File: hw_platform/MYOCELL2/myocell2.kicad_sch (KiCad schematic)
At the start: 22 parts, among them J1 Conn_01x16, J2 Conn_01x16, U1 ESP32-WROOM-32, U2 OPA340NA, U3 ADS1292, U4 OPA340NA

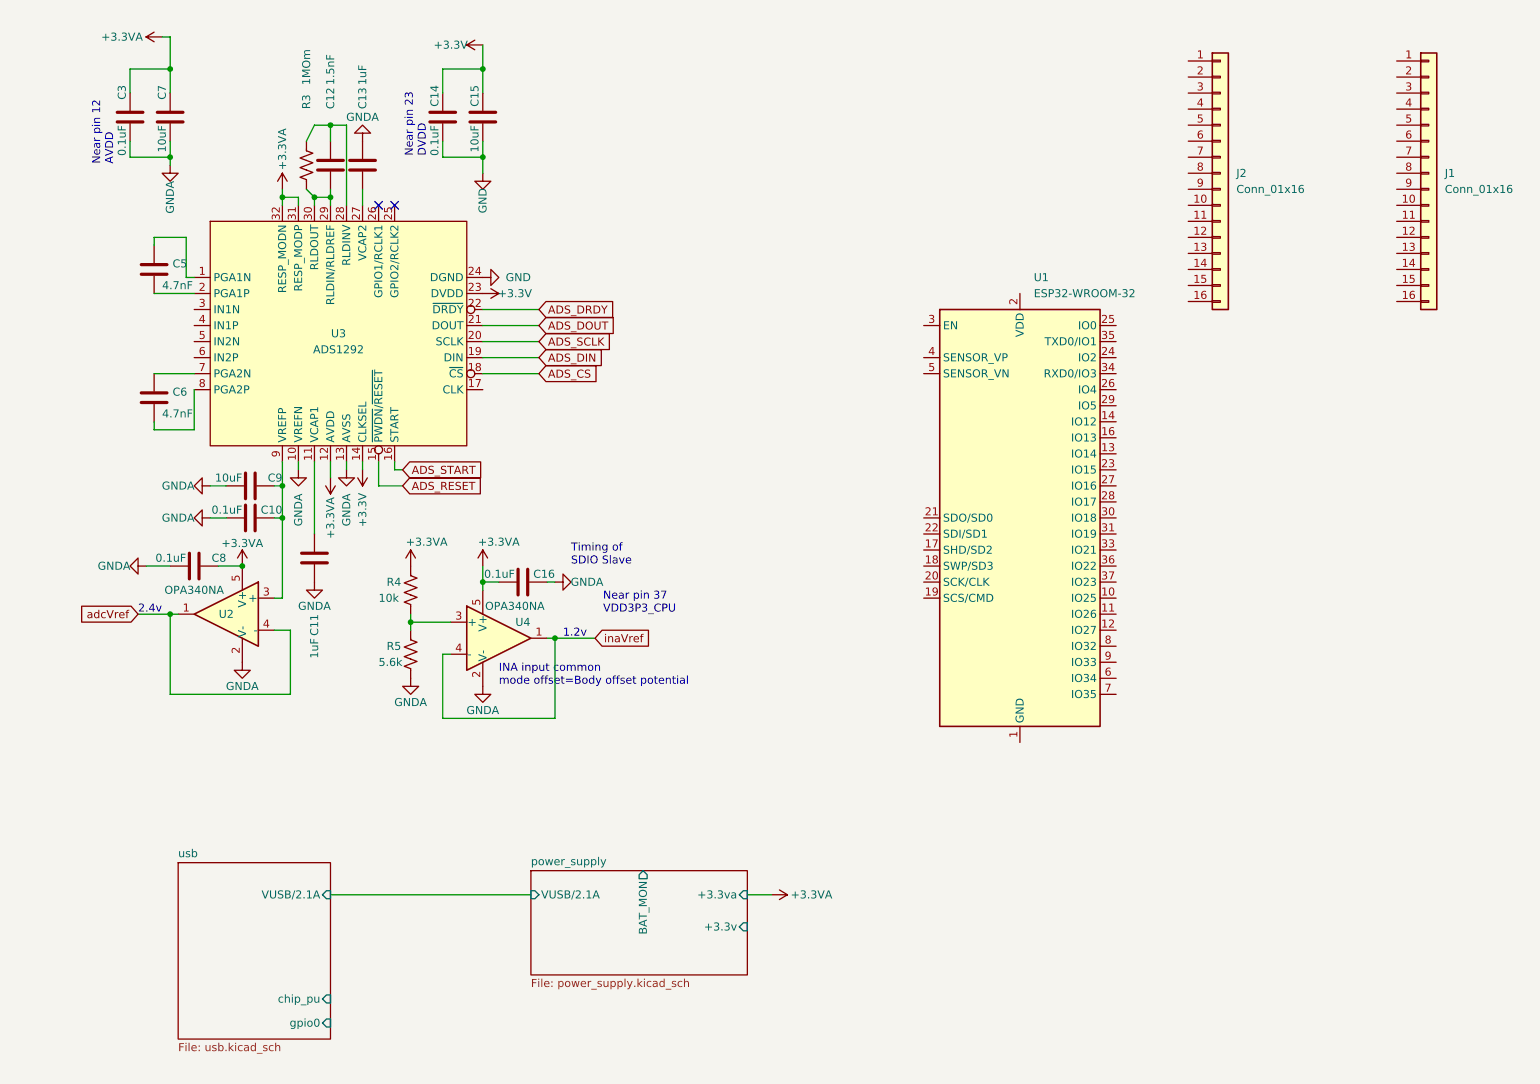
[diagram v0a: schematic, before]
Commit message: working on schematic:
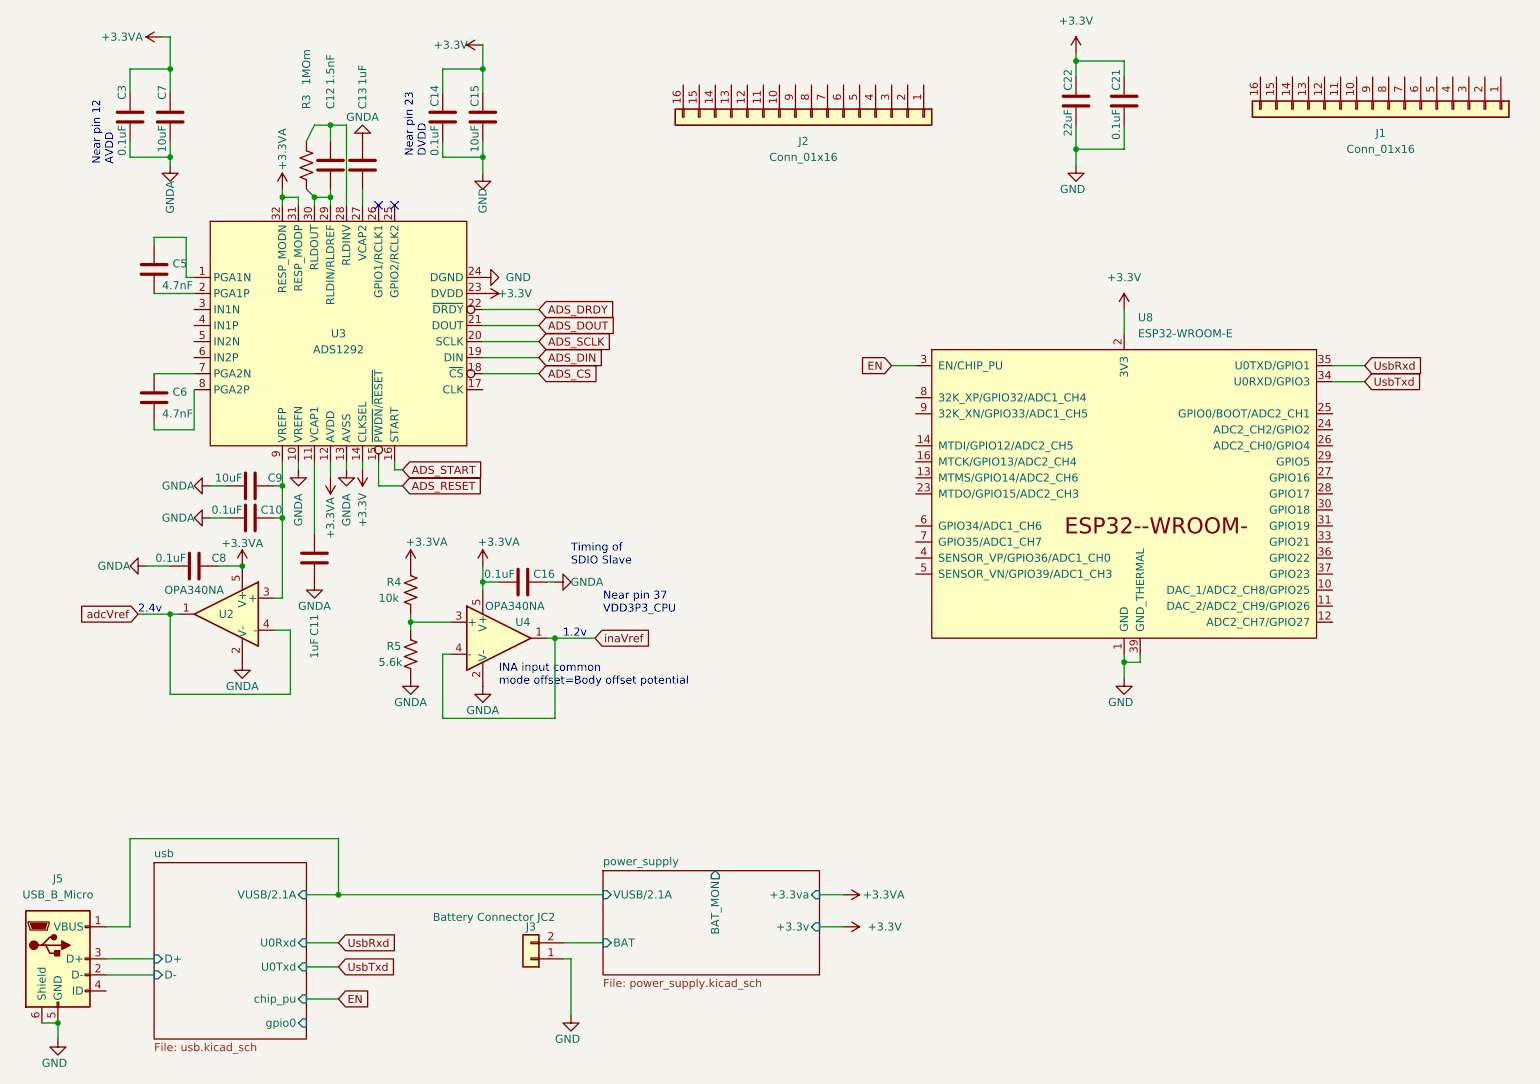
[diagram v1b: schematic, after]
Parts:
- removed U1: ESP32-WROOM-32, RF_Module:ESP32-WROOM-32, symbol RF_Module:ESP32-WROOM-32
- added C21: 0.1uF, Capacitor_SMD:C_0805_2012Metric_Pad1.18x1.45mm_HandSolder, symbol Device:C
- added C22: 22uF, Capacitor_SMD:C_0805_2012Metric_Pad1.18x1.45mm_HandSolder, symbol Device:C
- added J3: Battery Connector JC2, Connector_JST:JST_EH_B2B-EH-A_1x02_P2.50mm_Vertical, symbol Connector_Generic:Conn_01x02
- added J5: USB_B_Micro, Connector_USB:USB3_Micro-B_Connfly_DS1104-01, symbol Connector:USB_B_Micro
- added U8: ESP32-WROOM-E, PCM_Espressif:ESP32-WROOM-32E, symbol espressif_github:ESP32-WROOM-E
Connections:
- net +3.3V: now also C21.2, C22.2, U8.2 (3V3)
- net GND: now also C21.1, C22.1, J3.1 (Pin_1), J5.5 (GND), J5.6 (Shield), U8.1 (GND), U8.15 (GND), U8.38 (GND), U8.39 (GND_THERMAL)
- net power_supply/VUSB/2.1A: now also J5.1 (VBUS)
- new net EN: U8.3 (EN/CHIP_PU)
- new net UsbRxd: U8.35 (U0TXD/GPIO1)
- new net UsbTxd: U8.34 (U0RXD/GPIO3)
- new net power_supply/BAT: J3.2 (Pin_2)
- new net usb/D+: J5.3 (D+)
- new net usb/D-: J5.2 (D-)
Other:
- sheet power_supply ports: added BAT; removed none
- sheet usb ports: added D+, D-, U0Rxd, U0Txd; removed none
- moved on the sheet: J1, J2
